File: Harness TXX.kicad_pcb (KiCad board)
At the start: 2 copper layers, 88.7 x 50.8 mm, 67 parts, among them J1 DEUTSCH DT Inp, J2 DEUTSCH DT Data, J3 DEUTSCH DT Out, J4 Conn_01x02, J6 SWD, SW1 CAS-120B, SW2 CAS-120B, SW3 SW_SPDT, U1 LMR51420, U2 AMS1117-3.3, U3 STM32F105RCTx, U4 SN65HVD230, Y1 16MHz

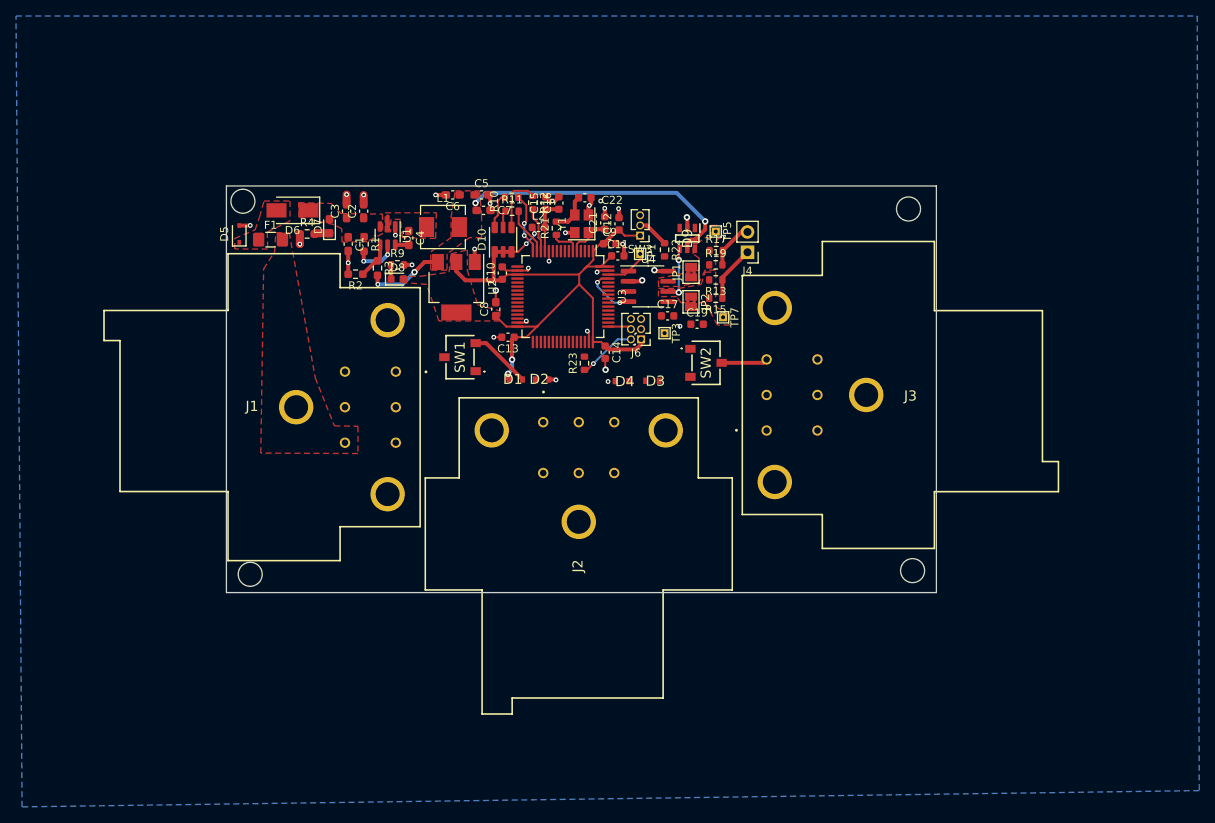
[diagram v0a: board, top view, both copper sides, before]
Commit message: Had been modifying a file on my computer and not git on accident. Adding updated PCB to Git
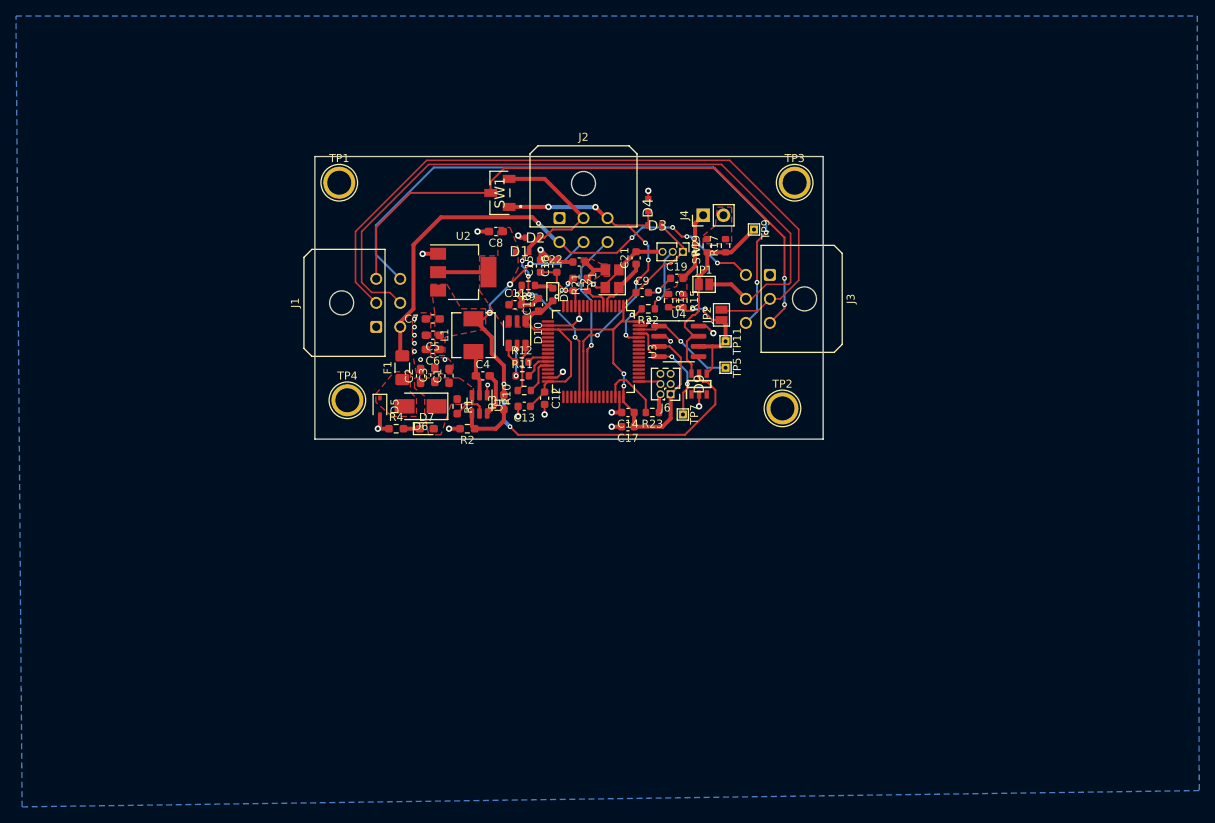
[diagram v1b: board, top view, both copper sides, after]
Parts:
- removed the SW2 at (106.8, 95.9)
- added G***: LOGO, custom symbols:flaggers, B.Cu at (88.6, 90.9)
- added TP1: TestPoint, TestPoint:TestPoint_Plated_Hole_D3.0mm, F.Cu at (61.0, 73.4)
- added TP2: TestPoint, TestPoint:TestPoint_Plated_Hole_D3.0mm, F.Cu at (116.3, 101.6)
- added TP3: TestPoint, TestPoint:TestPoint_Plated_Hole_D3.0mm, F.Cu at (117.9, 73.4)
- added TP4: TestPoint, TestPoint:TestPoint_Plated_Hole_D3.0mm, F.Cu at (62.0, 100.6)
- J1, J2, J3: footprint Global Libraries:DT13-6P -> Connector_Molex:Molex_Micro-Fit_3.0_43045-0600_2x03_P3.00mm_Horizontal
- SW1: value CAS-120B -> SW_SPDT; footprint SamacSys_Parts:CAS120B -> SamacSys_Parts:CAS120A1
- moved D6 29.3 mm to (71.1, 101.3)
- moved D7 28.1 mm to (71.9, 104.1), turned to 0 degrees
- moved D5 27.8 mm to (66.0, 101.3), turned to -90 degrees
- moved R4 26.8 mm to (68.1, 104.1)
- moved R10 24.2 mm to (84.1, 99.4)
- moved U1 24.0 mm to (78.5, 101.1)
- moved R2 23.8 mm to (77.0, 104.1)
- moved C12 23.7 mm to (86.6, 100.3), turned to -90 degrees
- moved R1 23.4 mm to (75.7, 101.3)
- moved C3 23.3 mm to (72.9, 97.4)
- moved R3 23.0 mm to (81.5, 100.8), turned to 90 degrees
- moved F1 23.0 mm to (68.8, 96.5), turned to 90 degrees
- moved J2 22.6 mm to (88.5, 77.8), turned to 0 degrees
- moved D4 22.2 mm to (99.6, 76.2), turned to 90 degrees
- moved C2 21.8 mm to (71.1, 97.5)
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- renumbered SW3 to SW2, TP7 to TP11, TP1 to TP5, TP3 to TP7, TP5 to TP9
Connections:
- J1 pad 3: /PassThru1 -> /PassThru
- J3 pad 3: /PassThru2 -> /PassThru
- SW1 pad 2: /PassThru1 -> /PassThru
- U3 pad 14: /MCU/LED_R -> /MCU/PB0
- U3 pad 15: /MCU/LED_G -> /MCU/PB1
- U3 pad 16: /MCU/LED_B -> /MCU/PB2
- U3 pad 26: /MCU/PB0 -> /MCU/LED_R
- U3 pad 27: /MCU/PB1 -> /MCU/LED_G
- U3 pad 28: /MCU/PB2 -> /MCU/LED_B
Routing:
- net /CAN+: track 0.00 -> 90.7 mm
- net /CAN-: track 0.00 -> 90.3 mm
- net /PassThru: track 0.00 -> 76.4 mm, vias 0 -> 2
- net /SHIELD: track 0.00 -> 76.3 mm, vias 0 -> 2
- net +24V: track 0.00 -> 63.2 mm, vias 0 -> 5
- net /WheelIn1: track 0.00 -> 46.4 mm, vias 0 -> 6
- net /WheelIn2: track 7.74 -> 42.3 mm, vias 0 -> 4
- net Net-(D9-Pad6): track 0.00 -> 25.9 mm
- net +5V: track 45.2 -> 67.7 mm, vias 4 -> 5
- net /Extra1: track 0.00 -> 21.5 mm, vias 0 -> 1
- net GND: track 44.5 -> 60.4 mm, vias 31 -> 28
- net Net-(D9-Pad4): track 5.50 -> 17.7 mm
- net /MCU/SWDIO: track 0.00 -> 8.21 mm
- net +3V3: track 83.2 -> 91.1 mm
- net /MCU/CAN1_RX: track 6.83 -> 14.6 mm
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- added copper zone on F.Cu, net GND
- added copper zone on F.Cu, net Net-(C19-Pad2)
- added copper zone on F.Cu, net Net-(C22-Pad1)
- added copper zone on F.Cu, net Net-(J4-Pad2)
- removed copper zone on F.Cu, net +24V
- removed copper zone on F.Cu, net /VRM/BUCK/SW
- removed copper zone on F.Cu, net Net-(D9-Pad4)
- removed copper zone on F.Cu, net Net-(D9-Pad6)
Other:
- board size 88.7 x 50.8 mm -> 63.5 x 35.3 mm
